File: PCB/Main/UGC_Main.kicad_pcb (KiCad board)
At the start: 2 copper layers, 125.7 x 77 mm, 19 parts, among them J1 Rumble, J2 LT, J3 RT, J4 UJ31-CH-G1-SMT-TR, SW1 SW_Push, SW10 SW_Push, SW11 SW_Push, SW12 SW_Push, SW13 SW_Push, SW2 SW_Push, SW3 SW_Push, SW4 SW_Push, SW5 SW_Push, SW6 GL18_SW, SW7 SW_Push, SW8 SW_Push, SW9 TS09-63-25-R-260-SMT

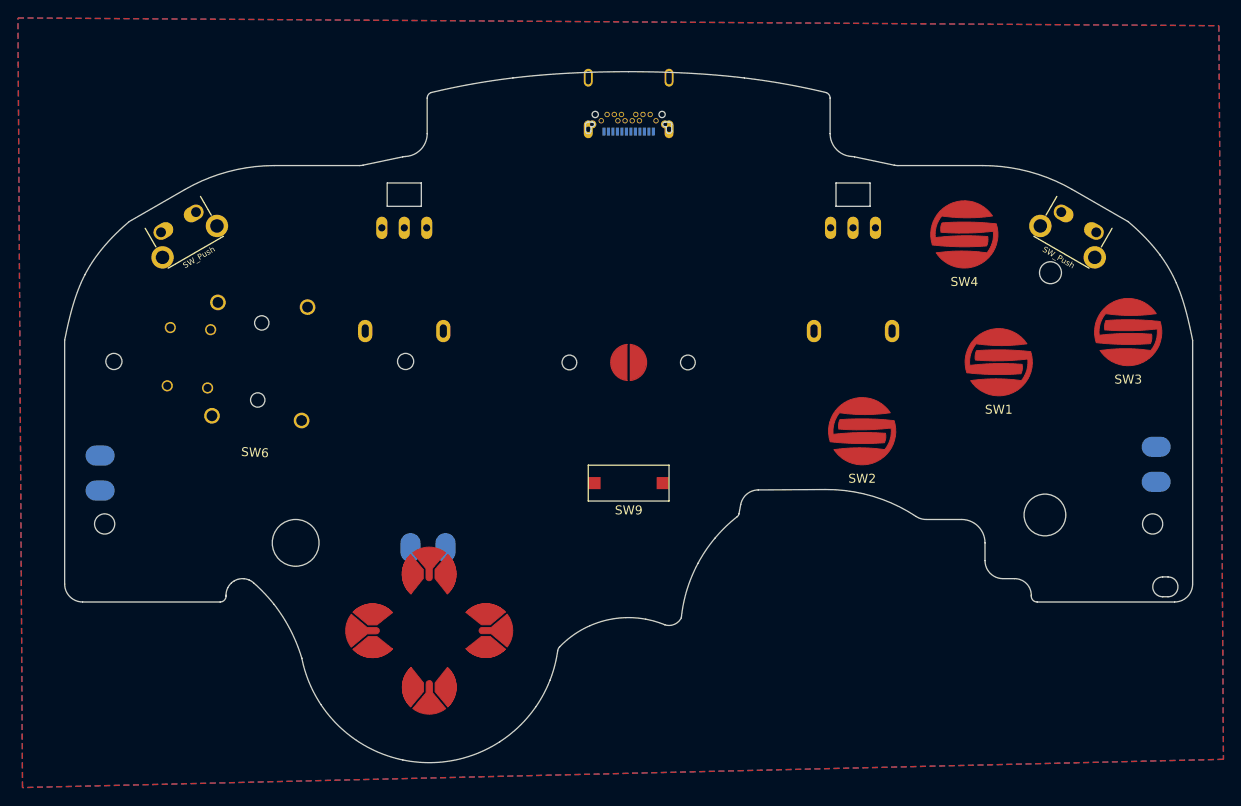
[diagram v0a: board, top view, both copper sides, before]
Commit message: Update shell and PCB
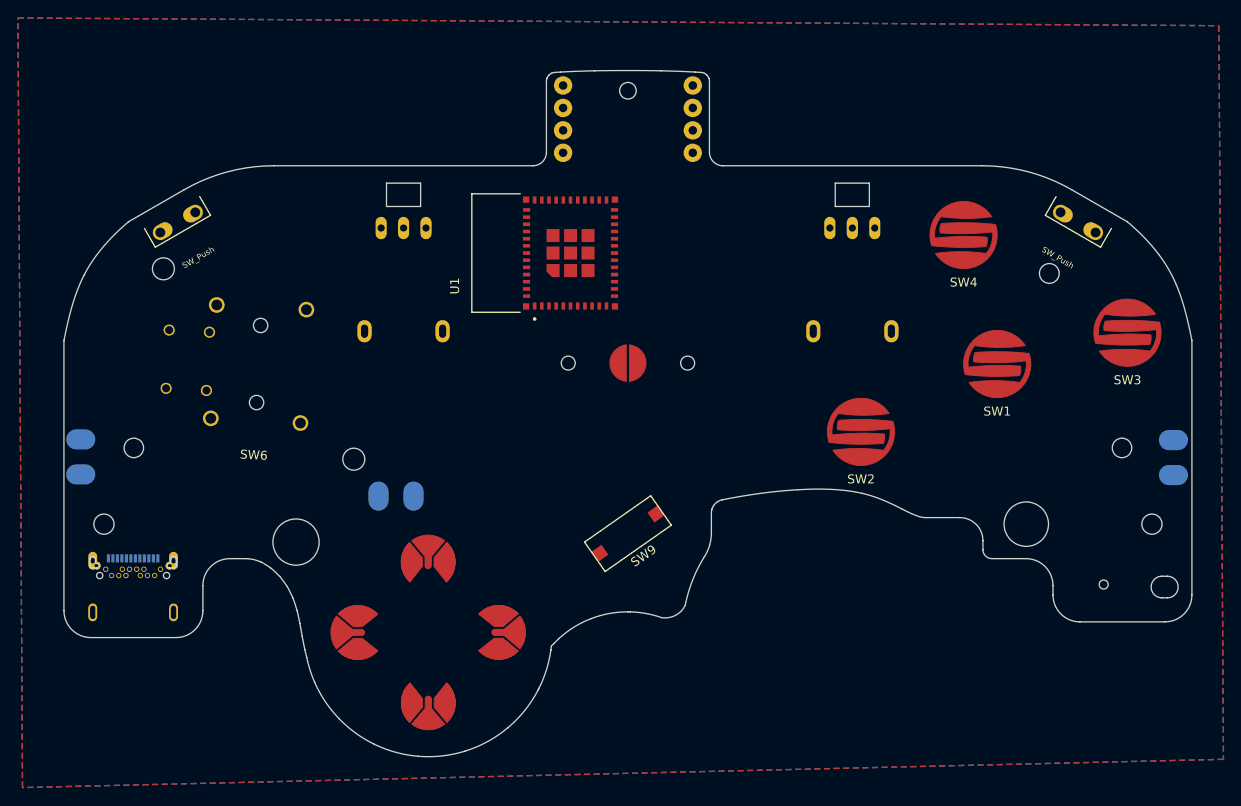
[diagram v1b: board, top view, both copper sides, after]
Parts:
- added J10: Conn_01x01_Pin, hhl:YZ72015053P-01, F.Cu at (225.7, 90.6)
- added J11: Conn_01x01_Pin, hhl:YZ72015053P-01, F.Cu at (211.3, 93.1)
- added J12: Conn_01x01_Pin, hhl:YZ72015053P-01, F.Cu at (225.7, 93.1)
- added J5: Conn_01x01_Pin, hhl:YZ72015053P-01, F.Cu at (211.3, 85.6)
- added J6: Conn_01x01_Pin, hhl:YZ72015053P-01, F.Cu at (225.7, 85.6)
- added J7: Conn_01x01_Pin, hhl:YZ72015053P-01, F.Cu at (211.3, 88.1)
- added J8: Conn_01x01_Pin, hhl:YZ72015053P-01, F.Cu at (225.7, 88.1)
- added J9: Conn_01x01_Pin, hhl:YZ72015053P-01, F.Cu at (211.3, 90.6)
- added U1: ESP32-PICO-MINI-02, hhl:MODULE_ESP32-PICO-MINI-02, F.Cu at (212.1, 104.2)
- moved J4 68.8 mm to (166.1, 138.2), turned to 180 degrees
- moved J1 6.76 mm to (193.8, 131.3)
- moved SW9 5.63 mm to (218.5, 135.5), turned to 35 degrees
- moved J2 4.64 mm to (157.5, 125.8), turned to 180 degrees
- moved J3 2.46 mm to (279.2, 128.2), turned to 0 degrees
- moved SW11 1.74 mm to (196.2, 154.3)
- moved SW12 1.66 mm to (188.4, 146.5)
- moved SW13 1.44 mm to (204.1, 146.5)
- moved SW10 1.34 mm to (196.2, 138.6)
- moved SW6 0.31 mm to (177.3, 116.6)
- moved SW1 0.27 mm to (259.6, 116.6)
- moved SW2 0.15 mm to (244.5, 124.1)
- moved SW3 0.11 mm to (274.1, 113.1)
- moved SW4 0.11 mm to (255.9, 102.2)
- moved SW5 0.11 mm to (218.5, 116.5)
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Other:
- board size 125.7 x 77 mm -> 125.7 x 76.4 mm
